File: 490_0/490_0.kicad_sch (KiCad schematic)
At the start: 37 parts, among them J1 DF40C-100DS-0.4V_51_, J2 DF40C-100DS-0.4V_51_, J3 Micro_SD_Card, J4 USB_A, J5 USB_C_Receptacle, Q1 NMOS, SW1 SW_DPST_x2, U1 RT9742GGJ5, U2 MCP73832-2-OT

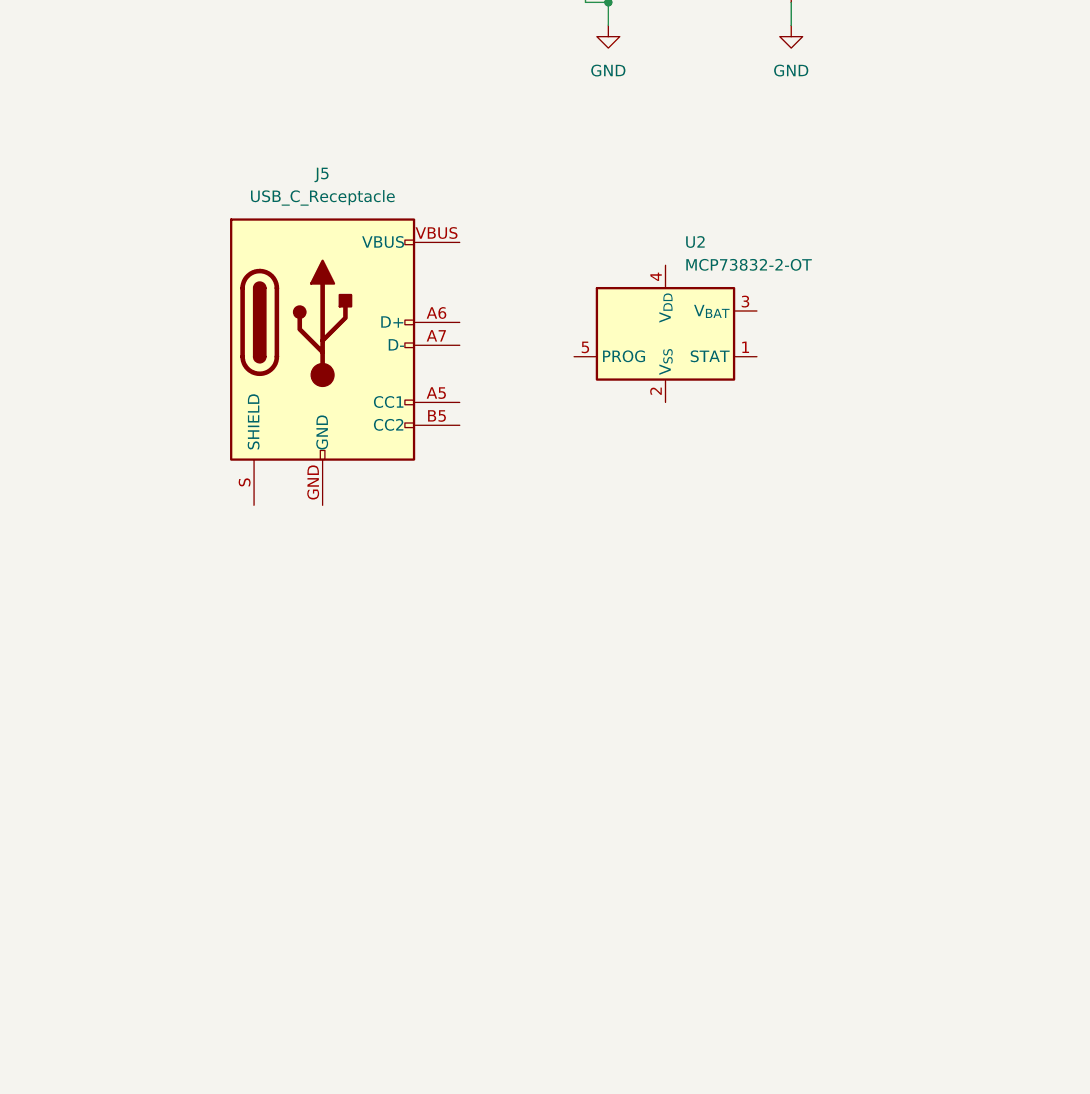
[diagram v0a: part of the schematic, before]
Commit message: Startted power
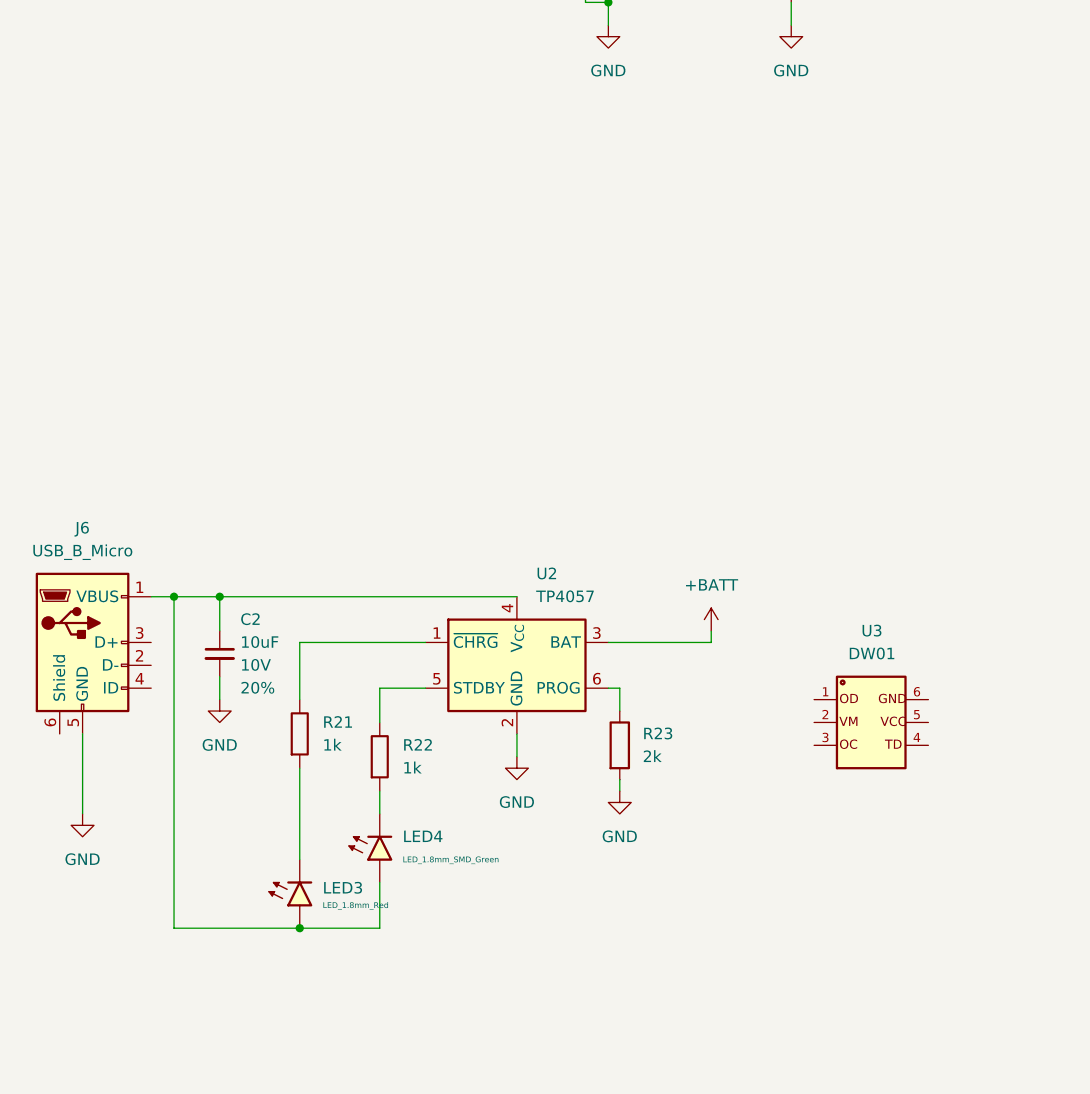
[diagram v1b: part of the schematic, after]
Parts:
- removed J5: USB_C_Receptacle, PCM_SparkFun-Connector:USB-C_16, symbol PCM_SparkFun-Connector:USB_C_Receptacle
- removed U2: MCP73832-2-OT, Package_TO_SOT_SMD:SOT-23-5, symbol Battery_Management:MCP73832-2-OT
- added C2: 10uF, PCM_SparkFun-Capacitor:C_0603_1608Metric, symbol PCM_SparkFun-Capacitor:10uF_0603_10V_20%
- added J6: USB_B_Micro, symbol Connector:USB_B_Micro
- added LED3: LED_1.8mm_Red, PCM_LED_THT_AKL:LED_D1.8mm_W3.3mm_H2.4mm, symbol PCM_LED_AKL:LED_1.8mm_Red
- added LED4: LED_1.8mm_SMD_Green, PCM_LED_SMD_AKL:LED_1.8mm_GullWing, symbol PCM_LED_AKL:LED_1.8mm_SMD_Green
- added R21, R22: 1k, Resistor_THT:R_Axial_DIN0207_L6.3mm_D2.5mm_P10.16mm_Horizontal, symbol PCM_SL_Resistors:1k
- added R23: 2k_0603, 4ms_Resistor:R_0603, symbol PCM_4ms_Resistor:2k_0603
- added U2: TP4057, Package_TO_SOT_SMD:TSOT-23-6, symbol Battery_Management:TP4057
- added U3: DW01, DW01:SOT23-6, symbol capstone_parts:DW01
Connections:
- net GND: now also C2.2, J6.5 (GND), R23.2, U2.2 (GND)
- new net: R21.2, U2.1 (~{CHRG})
- new net: C2.1, J6.1 (VBUS), LED3.2 (A), LED4.2 (A), U2.4 (V_{CC})
- new net: R22.2, U2.5 (STDBY)
- new net: R23.1, U2.6 (PROG)
- new net: LED3.1 (K), R21.1
- new net: LED4.1 (K), R22.1
- new net +BATT: U2.3 (BAT)
